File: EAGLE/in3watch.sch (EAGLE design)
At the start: 297 parts, among them IC1 74HC595D, IC2 74HC595D, IC3 74HC595D, IC4 74HC595D, IC5 74HC595D, IC6 74HC595D, IC7 74HC595D, J3 J5MM

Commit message: ..
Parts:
- R75: device rcl:R-EU_R0805 -> rcl:R-EU_R1206W
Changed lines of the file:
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@@
 <grid distance="100" unitdist="mil" unit="mil" style="lines" multiple="1" display="yes" altdistance="0.01" altunitdist="inch" altunit="inch"/>
 <layers>
-<layer number="1" name="Top" color="4" fill="1" visible="no" active="no"/>
-<layer number="2" name="Route2" color="1" fill="3" visible="no" active="no"/>
-<layer number="3" name="Route3" color="4" fill="3" visible="no" active="no"/>
-<layer number="4" name="Route4" color="1" fill="4" visible="no" active="no"/>
-<layer number="5" name="Route5" color="4" fill="4" visible="no" active="no"/>
-<layer number="6" name="Route6" color="1" fill="8" visible="no" active="no"/>
-<layer number="7" name="Route7" color="4" fill="8" visible="no" active="no"/>
-<layer number="8" name="Route8" color="1" fill="2" visible="no" active="no"/>
-<layer number="9" name="Route9" color="4" fill="2" visible="no" active="no"/>
-<layer number="10" name="Route10" color="1" fill="7" visible="no" active="no"/>
-<layer number="11" name="Route11" color="4" fill="7" visible="no" active="no"/>
-<layer number="12" name="Route12" color="1" fill="5" visible="no" active="no"/>
-<layer number="13" name="Route13" color="4" fill="5" visible="no" active="no"/>
-<layer number="14" name="Route14" color="1" fill="6" visible="no" active="no"/>
-<layer number="15" name="Route15" color="4" fill="6" visible="no" active="no"/>
-<layer number="16" name="Bottom" color="1" fill="1" visible="no" active="no"/>
-<layer number="17" name="Pads" color="2" fill="1" visible="no" active="no"/>
-<layer number="18" name="Vias" color="2" fill="1" visible="no" active="no"/>
-<layer number="19" name="Unrouted" color="6" fill="1" visible="no" active="no"/>
-<layer number="20" name="Dimension" color="15" fill="1" visible="no" active="no"/>
-<layer number="21" name="tPlace" color="7" fill="1" visible="no" active="no"/>
-<layer number="22" name="bPlace" color="7" fill="1" visible="no" active="no"/>
-<layer number="23" name="tOrigins" color="15" fill="1" visible="no" active="no"/>
-<layer number="24" name="bOrigins" color="15" fill="1" visible="no" active="no"/>
-<layer number="25" name="tNames" color="7" fill="1" visible="no" active="no"/>
-<layer number="26" name="bNames" color="7" fill="1" visible="no" active="no"/>
-<layer number="27" name="tValues" color="7" fill="1" visible="no" active="no"/>
-<layer number="28" name="bValues" color="7" fill="1" visible="no" active="no"/>
+<layer number="1" name="Top" color="4" fill="1" visible="yes" active="no"/>
+<layer number="2" name="Route2" color="1" fill="3" visible="yes" active="no"/>
+<layer number="3" name="Route3" color="4" fill="3" visible="yes" active="no"/>
+<layer number="4" name="Route4" color="1" fill="4" visible="yes" active="no"/>
+<layer number="5" name="Route5" color="4" fill="4" visible="yes" active="no"/>
+<layer number="6" name="Route6" color="1" fill="8" visible="yes" active="no"/>
+<layer number="7" name="Route7" color="4" fill="8" visible="yes" active="no"/>
+<layer number="8" name="Route8" color="1" fill="2" visible="yes" active="no"/>
+<layer number="9" name="Route9" color="4" fill="2" visible="yes" active="no"/>
+<layer number="10" name="Route10" color="1" fill="7" visible="yes" active="no"/>
+<layer number="11" name="Route11" color="4" fill="7" visible="yes" active="no"/>
+<layer number="12" name="Route12" color="1" fill="5" visible="yes" active="no"/>
+<layer number="13" name="Route13" color="4" fill="5" visible="yes" active="no"/>
+<layer number="14" name="Route14" color="1" fill="6" visible="yes" active="no"/>
+<layer number="15" name="Route15" color="4" fill="6" visible="yes" active="no"/>
+<layer number="16" name="Bottom" color="1" fill="1" visible="yes" active="no"/>
+<layer number="17" name="Pads" color="2" fill="1" visible="yes" active="no"/>
+<layer number="18" name="Vias" color="2" fill="1" visible="yes" active="no"/>
+<layer number="19" name="Unrouted" color="6" fill="1" visible="yes" active="no"/>
+<layer number="20" name="Dimension" color="15" fill="1" visible="yes" active="no"/>
+<layer number="21" name="tPlace" color="7" fill="1" visible="yes" active="no"/>
+<layer number="22" name="bPlace" color="7" fill="1" visible="yes" active="no"/>
+<layer number="23" name="tOrigins" color="15" fill="1" visible="yes" active="no"/>
+<layer number="24" name="bOrigins" color="15" fill="1" visible="yes" active="no"/>
+<layer number="25" name="tNames" color="7" fill="1" visible="yes" active="no"/>
+<layer number="26" name="bNames" color="7" fill="1" visible="yes" active="no"/>
+<layer number="27" name="tValues" color="7" fill="1" visible="yes" active="no"/>
+<layer number="28" name="bValues" color="7" fill="1" visible="yes" active="no"/>
 <layer number="29" name="tStop" color="7" fill="3" visible="no" active="no"/>
 <layer number="30" name="bStop" color="7" fill="6" visible="no" active="no"/>
@@
 <layer number="35" name="tGlue" color="7" fill="4" visible="no" active="no"/>
 <layer number="36" name="bGlue" color="7" fill="5" visible="no" active="no"/>
-<layer number="37" name="tTest" color="7" fill="1" visible="no" active="no"/>
-<layer number="38" name="bTest" color="7" fill="1" visible="no" active="no"/>
+<layer number="37" name="tTest" color="7" fill="1" visible="yes" active="no"/>
+<layer number="38" name="bTest" color="7" fill="1" visible="yes" active="no"/>
 <layer number="39" name="tKeepout" color="4" fill="11" visible="no" active="no"/>
 <layer number="40" name="bKeepout" color="1" fill="11" visible="no" active="no"/>
@@
 <layer number="44" name="Drills" color="7" fill="1" visible="no" active="no"/>
 <layer number="45" name="Holes" color="7" fill="1" visible="no" active="no"/>
-<layer number="46" name="Milling" color="3" fill="1" visible="no" active="no"/>
-<layer number="47" name="Measures" color="7" fill="1" visible="no" active="no"/>
-<layer number="48" name="Document" color="7" fill="1" visible="no" active="no"/>
-<layer number="49" name="Reference" color="7" fill="1" visible="no" active="no"/>
-<layer number="50" name="dxf" color="7" fill="1" visible="no" active="no"/>
-<layer number="51" name="tDocu" color="15" fill="1" visible="no" active="no"/>
-<layer number="52" name="bDocu" color="7" fill="1" visible="no" active="no"/>
-<layer number="53" name="tGND_GNDA" color="7" fill="9" visible="no" active="no"/>
-<layer number="54" name="bGND_GNDA" color="1" fill="9" visible="no" active="no"/>
-<layer number="56" name="wert" color="7" fill="1" visible="no" active="no"/>
-<layer number="57" name="tCAD" color="7" fill="1" visible="no" active="no"/>
-<layer number="59" name="tCarbon" color="7" fill="1" visible="no" active="no"/>
-<layer number="60" name="bCarbon" color="7" fill="1" visible="no" active="no"/>
+<layer number="46" name="Milling" color="3" fill="1" visible="yes" active="no"/>
+<layer number="47" name="Measures" color="7" fill="1" visible="yes" active="no"/>
+<layer number="48" name="Document" color="7" fill="1" visible="yes" active="no"/>
+<layer number="49" name="Reference" color="7" fill="1" visible="yes" active="no"/>
+<layer number="50" name="dxf" color="7" fill="1" visible="yes" active="no"/>
+<layer number="51" name="tDocu" color="15" fill="1" visible="yes" active="no"/>
+<layer number="52" name="bDocu" color="7" fill="1" visible="yes" active="no"/>
+<layer number="53" name="tGND_GNDA" color="7" fill="9" visible="yes" active="no"/>
+<layer number="54" name="bGND_GNDA" color="1" fill="9" visible="yes" active="no"/>
+<layer number="56" name="wert" color="7" fill="1" visible="yes" active="no"/>
+<layer number="57" name="tCAD" color="7" fill="1" visible="yes" active="no"/>
+<layer number="59" name="tCarbon" color="7" fill="1" visible="yes" active="no"/>
+<layer number="60" name="bCarbon" color="7" fill="1" visible="yes" active="no"/>
 <layer number="90" name="Modules" color="5" fill="1" visible="yes" active="yes"/>
 <layer number="91" name="Nets" color="2" fill="1" visible="yes" active="yes"/>
@@
 <part name="VD37" library="diode" deviceset="ZENER-DIODE" device="SOD80C"/>
 <part name="VT38" library="transistor-npn" deviceset="BC849*" device="SMD" value=""/>
-<part name="R75" library="rcl" deviceset="R-EU_" device="R0805"/>
+<part name="R75" library="rcl" deviceset="R-EU_" device="R1206W"/>
 <part name="R76" library="rcl" deviceset="R-EU_" device="0207/12"/>
 <part name="GND44" library="supply1" deviceset="GND" device=""/>

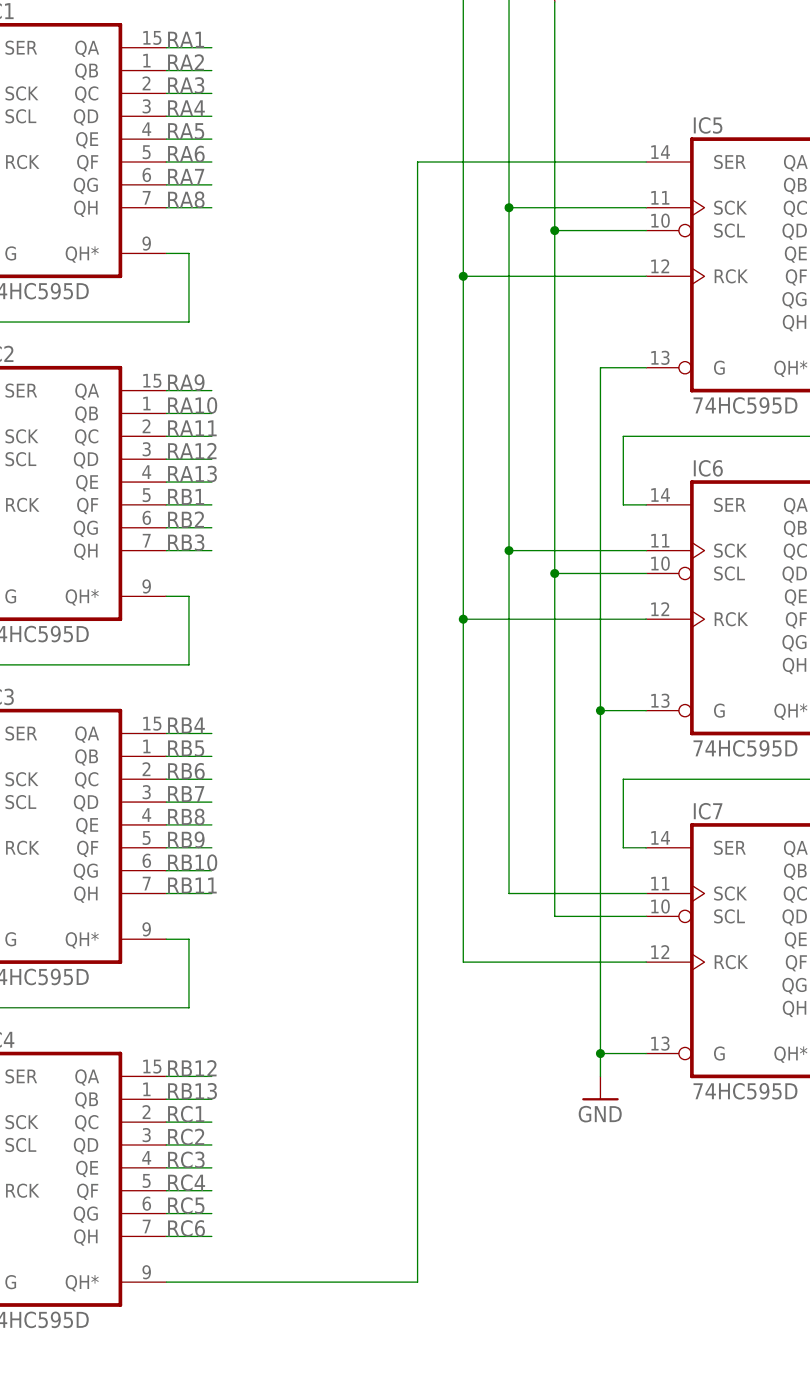
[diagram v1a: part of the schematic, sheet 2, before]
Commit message: ...
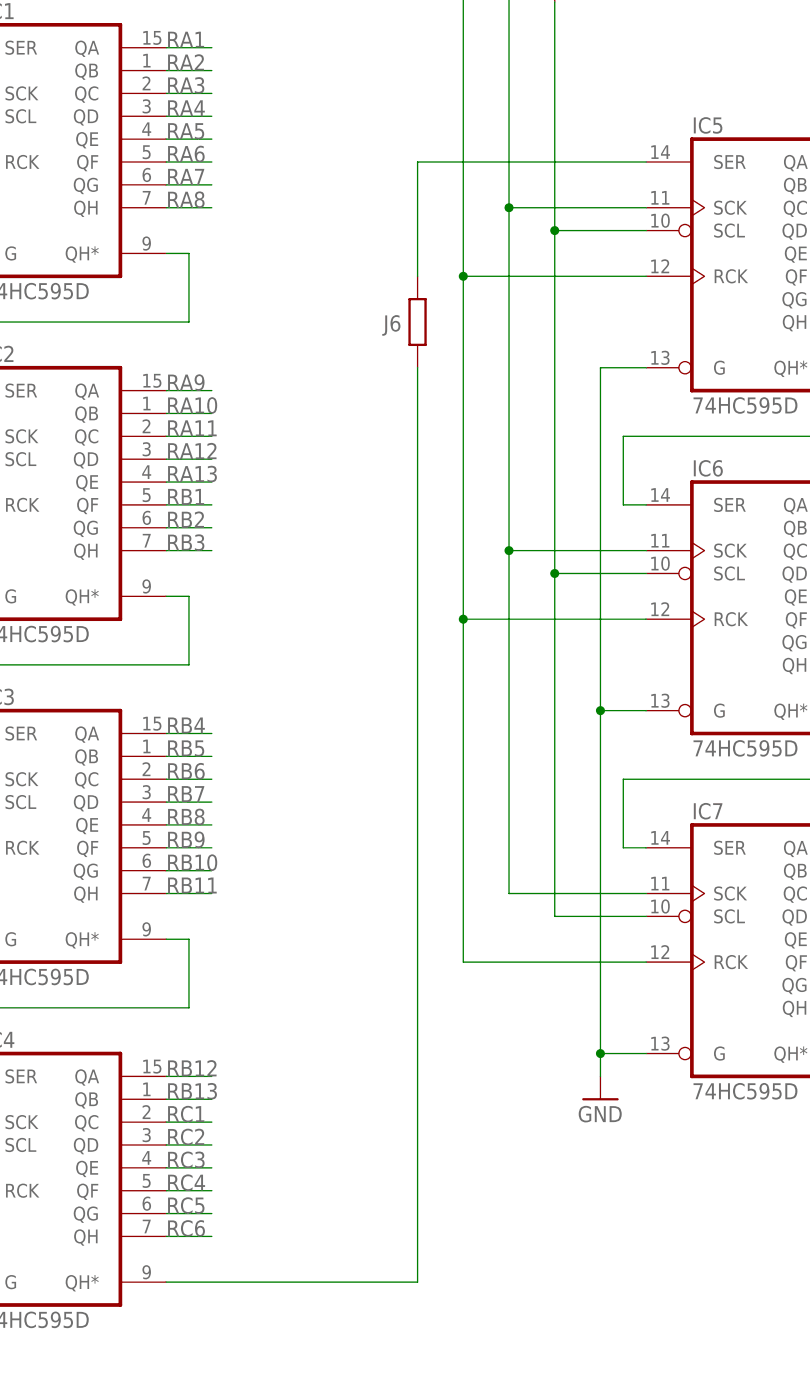
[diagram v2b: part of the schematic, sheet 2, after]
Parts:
- added J6: (no value), rcl:R-EU_R1206W
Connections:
- new net N$17: IC5A.SER, J6.2
- net SER5: now also J6.1; no longer IC5A.SER
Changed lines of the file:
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@@
 <part name="R110" library="rcl" deviceset="R-EU_" device="R0805" value="10k"/>
 <part name="R113" library="rcl" deviceset="R-EU_" device="R0805" value="10k"/>
+<part name="J6" library="rcl" deviceset="R-EU_" device="R1206W"/>
 </parts>
 <sheets>
@@
 </instance>
 <instance part="GND17" gate="1" x="203.2" y="88.9"/>
+<instance part="J6" gate="G$1" x="119.38" y="129.54" smashed="yes" rot="R90">
+<attribute name="NAME" x="115.57" y="128.4986" size="1.778" layer="95"/>
+<attribute name="VALUE" x="122.682" y="125.73" size="1.778" layer="96" rot="R90"/>
+</instance>
 </instances>
 <busses>
@@
 <pinref part="IC4" gate="A" pin="QH*"/>
 <wire x1="91.44" y1="22.86" x2="119.38" y2="22.86" width="0.1524" layer="91"/>
-<pinref part="IC5" gate="A" pin="SER"/>
-<wire x1="119.38" y1="22.86" x2="119.38" y2="147.32" width="0.1524" layer="91"/>
-<wire x1="119.38" y1="147.32" x2="144.78" y2="147.32" width="0.1524" layer="91"/>
+<wire x1="119.38" y1="22.86" x2="119.38" y2="124.46" width="0.1524" layer="91"/>
+<pinref part="J6" gate="G$1" pin="1"/>
 </segment>
 </net>
@@
 </segment>
 </net>
+<net name="N$17" class="0">
+<segment>
+<pinref part="IC5" gate="A" pin="SER"/>
+<wire x1="119.38" y1="147.32" x2="144.78" y2="147.32" width="0.1524" layer="91"/>
+<wire x1="119.38" y1="134.62" x2="119.38" y2="147.32" width="0.1524" layer="91"/>
+<pinref part="J6" gate="G$1" pin="2"/>
+</segment>
+</net>
